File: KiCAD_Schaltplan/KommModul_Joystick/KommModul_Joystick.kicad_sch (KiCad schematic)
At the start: 46 parts, among them J1 66100411622, J2 618015231121, J3 691242510004, J4 691242510004, J5 612020235121, J6 696106003002, SW1 430182080816, SW3 472123010111, U1 STM32F303RETx, U2 SP3485EN, U3 SP3485EN, U4 TLV1117LV33DCYR, Y1 16 MHz

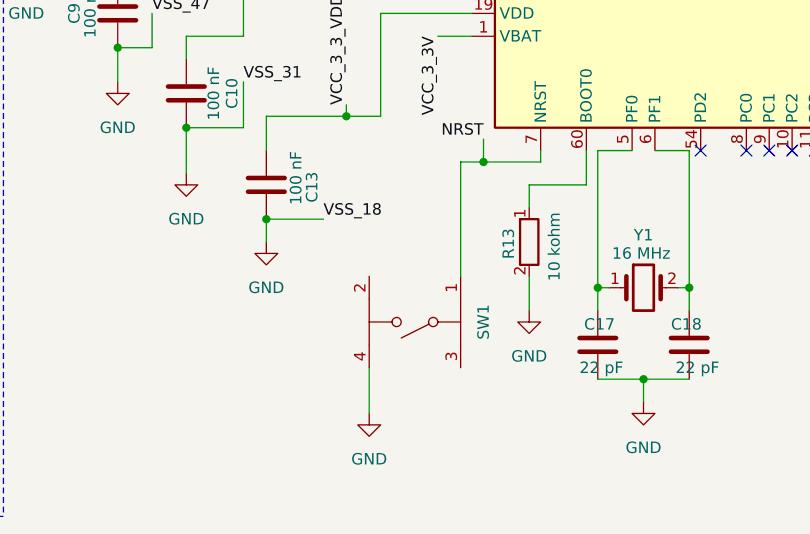
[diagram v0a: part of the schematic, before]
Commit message: PCB Layout V2
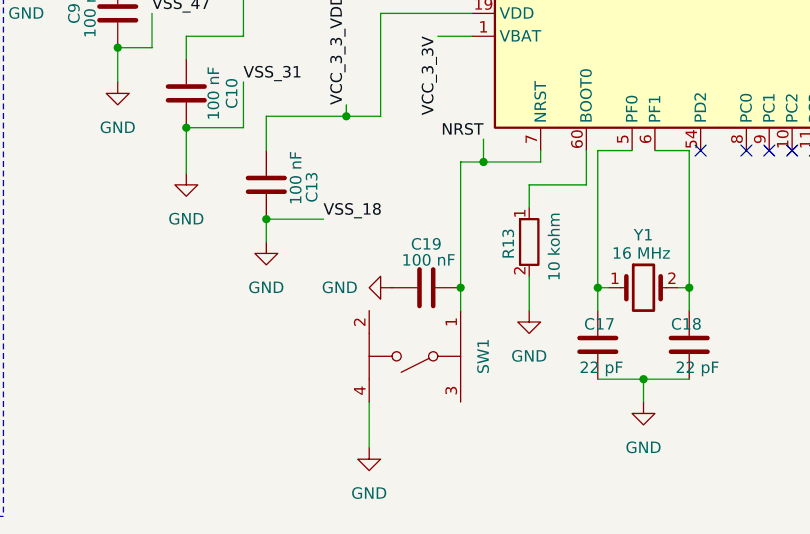
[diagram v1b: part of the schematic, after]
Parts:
- added C19: 100 nF, Capacitor_SMD_Wurth:C_Wurth_WCAP-CSGP-1206_H0.8, symbol symbols:1206_H0.8_885012208030
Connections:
- net GND: now also C19.2
- net NRST: now also C19.1
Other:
- moved on the sheet: SW1
